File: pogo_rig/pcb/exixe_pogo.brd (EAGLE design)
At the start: 100 x 80 mm, 14 parts, among them X1 USB-MICROB

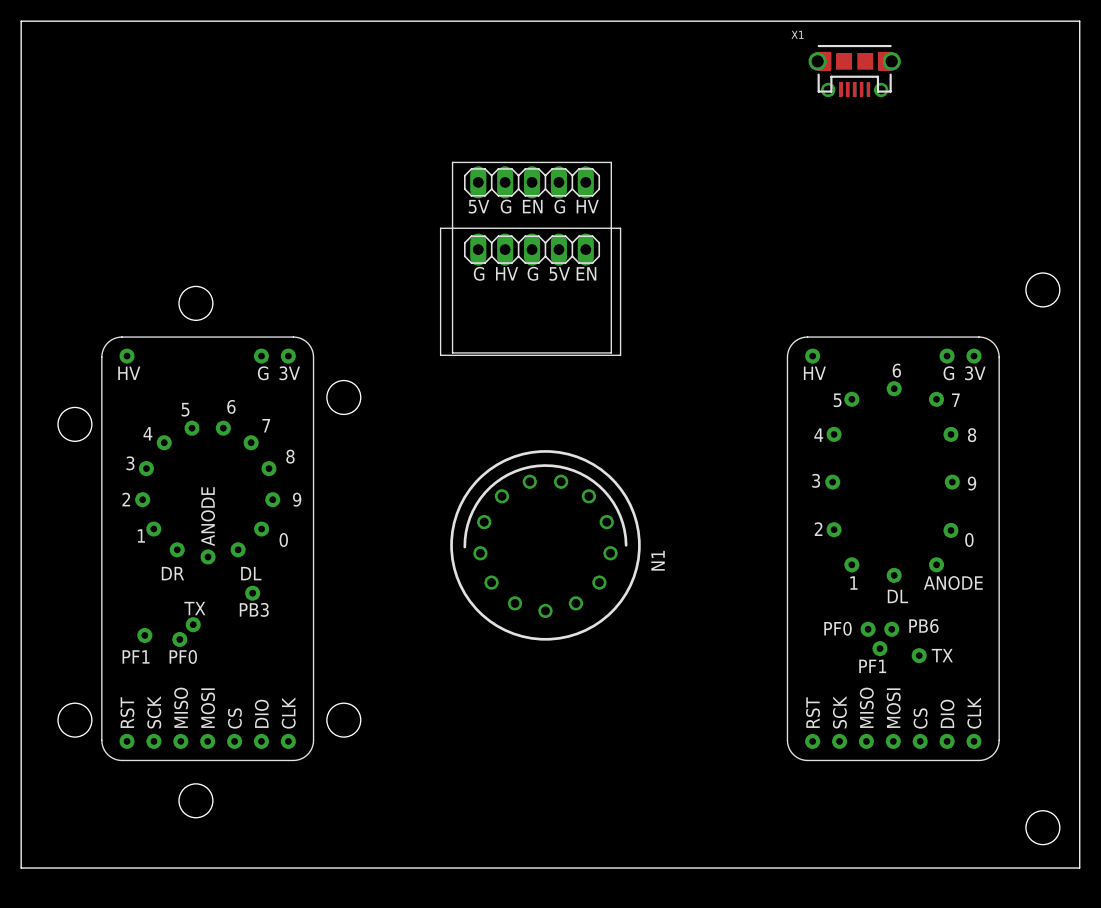
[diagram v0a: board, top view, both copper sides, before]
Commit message: working on pogo rig
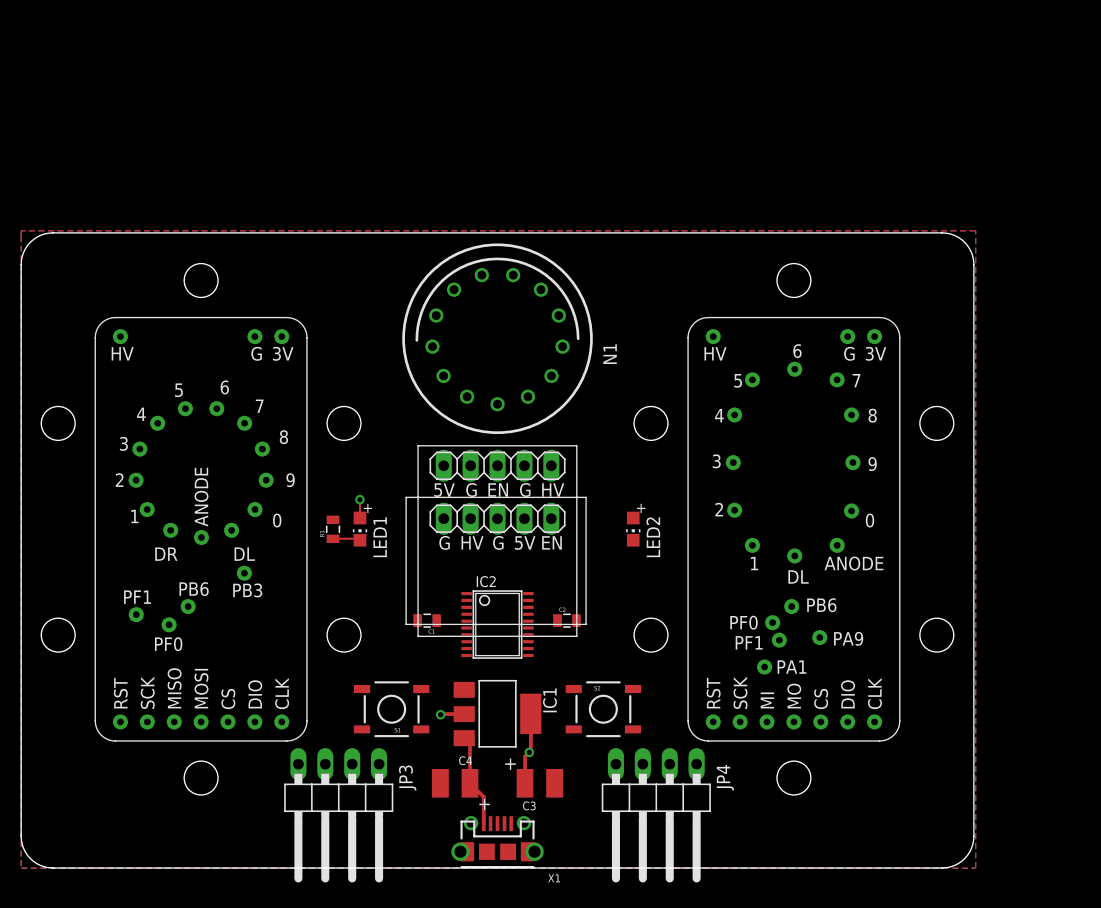
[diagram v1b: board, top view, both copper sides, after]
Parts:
- added C1, C2, R1: (no value), clock:0805
- added C3, C4: (no value), clock:C1210
- added IC1: REG1117, clock:SOT223
- added IC2: STM32F030F4, stm32f030f4:TSSOP20
- added JP3, JP4: (no value), clock:1X04/90
- added LED1, LED2: (no value), clock:CHIP-LED0805
- added S1, S2: TAC_SWITCHSMD, clock:TACTILE-SWITCH-SMD
- added U$11, U$12, U$13, U$14: M3_MOUNTING_HOLE, clock:M3_MOUNTING_HOLE_PACK
- moved X1 81.9 mm to (45.0, 1.54), turned to 0 degrees
- moved JP2 27.0 mm to (45.0, 38.0)
- moved JP1 25.6 mm to (45.0, 33.0)
- moved U$10 24.0 mm to (73.0, 8.50)
- moved U$8 23.5 mm to (73.0, 55.5)
- moved N1 20.0 mm to (45.0, 50.0)
- moved U$1 9.57 mm to (63.0, 12.0)
- moved U$4 8.18 mm to (3.50, 22.0)
- moved U$5 8.03 mm to (30.5, 22.0)
- moved U$6 2.45 mm to (30.5, 42.0)
- moved U$7 2.21 mm to (17.0, 55.5)
- moved U$9 2.21 mm to (17.0, 8.50)
- moved U$2 1.94 mm to (7.00, 12.0)
- moved U$3 1.58 mm to (3.50, 42.0)
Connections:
- new net +3V3: C1.1, C2.1, C3.1, IC1.2, IC1.4, IC2.16, IC2.5, JP3.2, JP4.2, LED1.A, U$1.3V, U$2.3V
- new net +5V: C4.1, IC1.3, X1.VBUS
- new net CS: IC2.10, U$1.CS, U$2.CS
- new net EXIXE_RST: U$1.RST, U$2.RST
- new net GND: C1.2, C2.2, C3.2, C4.2, IC1.1, IC2.1, IC2.15, JP3.1, JP4.1, R1.2, U$1.GND, U$2.GND, X1.GND, X1.P1, X1.P2, X1.P3, X1.P4, X1.P5, X1.P6
- new net MISO: IC2.12, U$1.MISO, U$2.MISO
- new net MOSI: IC2.13, U$1.MOSI, U$2.MOSI
- new net N$1: N1.1, U$1.DIGIT_1, U$2.DIGIT_1
- new net N$10: N1.9, U$1.DIGIT_9, U$2.DIGIT_9
- new net N$11: N1.0, U$1.DIGIT_0, U$2.DIGIT_0
- new net N$12: N1.RHDP, U$2.DOT_RIGHT
- new net N$13: N1.LHDP, U$1.DOT_LEFT, U$2.DOT_LEFT
- new net N$14: N1.A, U$1.ANODE, U$2.ANODE
- new net N$15: LED1.C, R1.1
- new net N$2: IC2.4, S1.3
- new net N$3: N1.2, U$1.DIGIT_2, U$2.DIGIT_2
- new net N$4: N1.3, U$1.DIGIT_3, U$2.DIGIT_3
- new net N$5: N1.4, U$1.DIGIT_4, U$2.DIGIT_4
- new net N$6: N1.5, U$1.DIGIT_5, U$2.DIGIT_5
- new net N$7: N1.6, U$1.DIGIT_6, U$2.DIGIT_6
- new net N$8: N1.7, U$1.DIGIT_7, U$2.DIGIT_7
- new net N$9: N1.8, U$1.DIGIT_8, U$2.DIGIT_8
- new net RX: IC2.9
- new net SCK: IC2.11, U$1.SCK, U$2.SCK
- new net SWCLK: IC2.20
- new net SWDIO: IC2.19
- new net TX: IC2.8
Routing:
- net +3V3: track 0.00 -> 10.8 mm, vias 0 -> 3
- net +5V: track 0.00 -> 8.83 mm
- net N$15: track 0.00 -> 2.60 mm
- added copper zone on layer 16, net +3V3
- added copper zone on layer 1, net GND
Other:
- board size 100 x 80 mm -> 90 x 60 mm
